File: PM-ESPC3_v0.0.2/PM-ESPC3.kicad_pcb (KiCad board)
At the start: 2 copper layers, 30.5 x 55.9 mm, 15 parts, among them J1 U254-051T-4BH83-S1S, J2 PinHeader_01x13_P2.54_THT_str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, J3 PinHeader_01x01_P2.54_THT_str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, SW1 Button, SW2 Button, SW3 DIP_SW-3P-P2.54-THT-Top, U1 ESP32-C3-WROOM-02U-N4

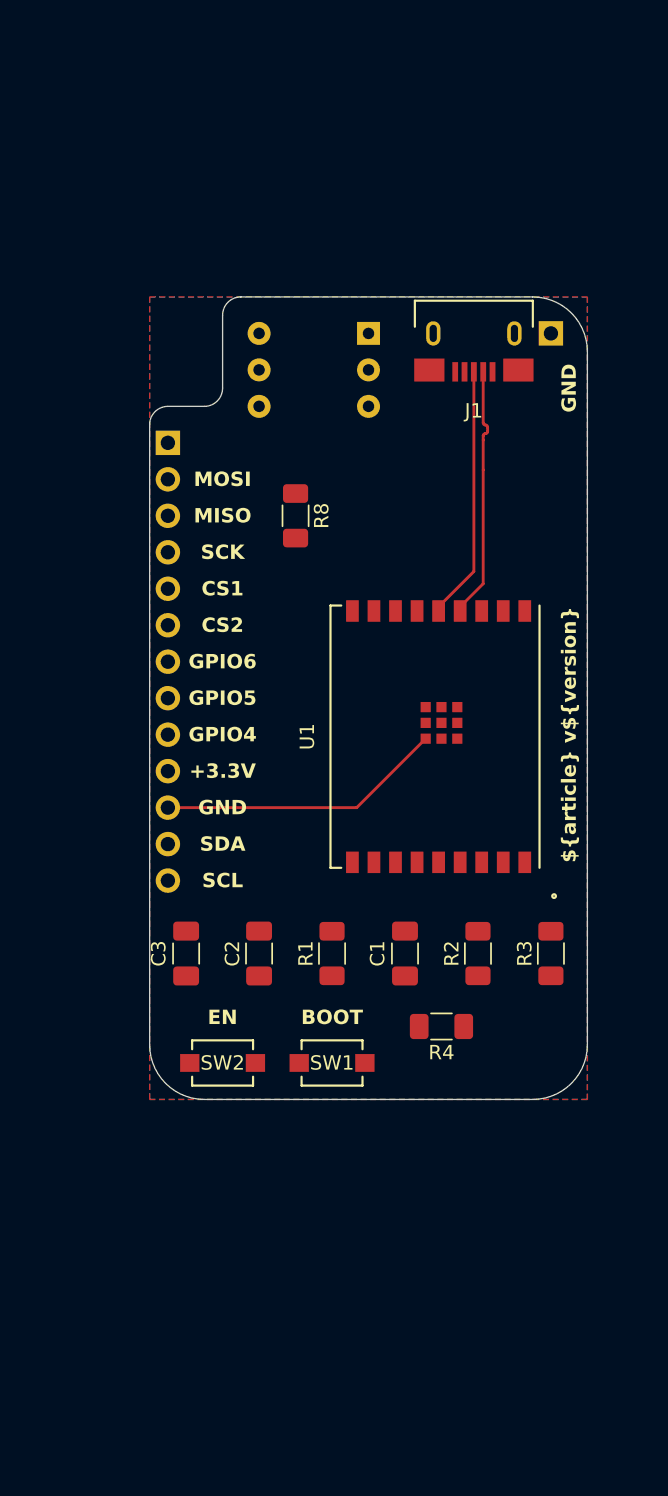
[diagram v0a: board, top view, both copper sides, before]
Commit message: new PM-RQ8
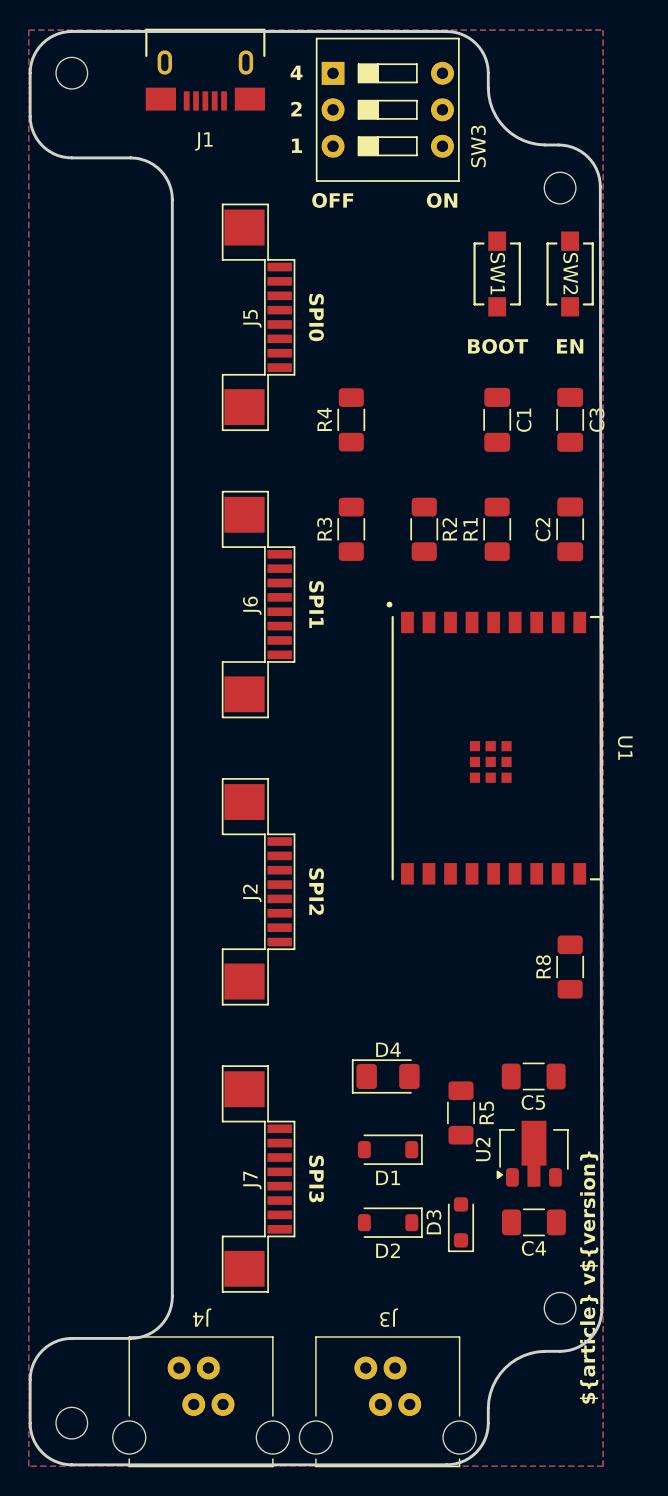
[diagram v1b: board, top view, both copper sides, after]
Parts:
- added C4: 10uF, Capacitor_SMD:C_1206_3216Metric_Pad1.33x1.80mm_HandSolder, F.Cu at (85.2, 133.0)
- added C5: 22uF, Capacitor_SMD:C_1206_3216Metric_Pad1.33x1.80mm_HandSolder, F.Cu at (85.2, 122.9)
- added D1: B5819W, Diode_SMD:D_SOD-123, F.Cu at (75.0, 128.0)
- added D2: B5819W, Diode_SMD:D_SOD-123, F.Cu at (75.0, 133.0)
- added D3: 5A 9.8V 6V, Diode_SMD:D_SOD-323_HandSoldering, F.Cu at (80.1, 133.0)
- added D4: Green, LED_SMD:LED_1206_3216Metric_Pad1.42x1.75mm_HandSolder, F.Cu at (75.0, 122.9)
- added H1: MountingHole, MountingHole:MountingHole_2.2mm_M2, F.Cu at (87.0, 139.0)
- added H2: MountingHole, MountingHole:MountingHole_2.2mm_M2, F.Cu at (53.0, 147.0)
- added H3: MountingHole, MountingHole:MountingHole_2.2mm_M2, F.Cu at (87.0, 61.0)
- added H4: MountingHole, MountingHole:MountingHole_2.2mm_M2, F.Cu at (53.0, 53.0)
- added J4: R-RJ11R04P-A802, kicad_inventree_lib:R-RJ11R04P-A802, F.Cu at (62.0, 148.0)
- added J5: X10B25L08T, kicad_inventree_lib:X10B25L08T, F.Cu at (67.5, 70.0)
- added J6: X10B25L08T, kicad_inventree_lib:X10B25L08T, F.Cu at (67.5, 90.0)
- added J7: X10B25L08T, kicad_inventree_lib:X10B25L08T, F.Cu at (67.5, 130.0)
- added R5: 680R, Resistor_SMD:R_1206_3216Metric_Pad1.30x1.75mm_HandSolder, F.Cu at (80.1, 125.4)
- added U2: CJA1117B-3.3, Package_TO_SOT_SMD:SOT-89-3, F.Cu at (85.2, 127.9)
- J2: value PinHeader_01x13_P2.54_THT_straight -> X10B25L08T; footprint Connector_PinHeader_2.54mm:PinHeader_1x13_P2.54mm_Vertical -> kicad_inventree_lib:X10B25L08T; moved to F.Cu
- J3: value PinHeader_01x01_P2.54_THT_straight -> R-RJ11R04P-A802; footprint Connector_PinHeader_2.54mm:PinHeader_1x01_P2.54mm_Vertical -> kicad_inventree_lib:R-RJ11R04P-A802; moved to F.Cu
- SW3: moved to F.Cu
- moved J3 77.7 mm to (75.0, 148.0)
- moved SW2 60.0 mm to (87.7, 67.0), turned to -90 degrees
- moved SW1 56.1 mm to (82.6, 67.0), turned to -90 degrees
- moved C3 45.8 mm to (87.7, 77.1), turned to 90 degrees
- moved R4 42.7 mm to (72.5, 77.1), turned to 90 degrees
- moved C1 37.7 mm to (82.6, 77.1), turned to 90 degrees
- moved R8 36.8 mm to (87.7, 115.2), turned to 90 degrees
- moved C2 36.6 mm to (87.7, 84.8)
- moved R3 32.6 mm to (72.5, 84.8)
- moved J2 32.2 mm to (67.5, 110.0), turned to -90 degrees
- moved R1 31.7 mm to (82.6, 84.8)
- moved R2 29.8 mm to (77.5, 84.8), turned to -90 degrees
- moved J1 26.6 mm to (63.6, 55.1)
- moved SW3 18.3 mm to (71.2, 53.0), turned to 0 degrees
- moved U1 4.40 mm to (82.6, 100.0), turned to -90 degrees
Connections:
- C2 pad 2: /+3.3V -> +3.3V
- C3 pad 1: /+3.3V -> +3.3V
- J1 pad 1: unconnected-(J1-VBUS-Pad1) -> Net-(D1-A)
- J2 pad 1: unconnected-(J2-Pin_1-Pad1) -> +5V
- J2 pad 2: /GPIO2 -> +3.3V
- J2 pad 3: /GPIO3 -> unconnected-(J2-Pin_3-Pad3)
- J2 pad 4: /GPIO9 -> /MOSI
- J2 pad 5: /GPIO8 -> /MISO
- J2 pad 6: /GPIO7 -> /SCK
- J2 pad 7: /GPIO6 -> /CS2
- J2 pad 8: /GPIO5 -> GND
- J3 pad 1: GND -> Net-(D2-A)
- R1 pad 1: /+3.3V -> +3.3V
- R2 pad 1: /+3.3V -> +3.3V
- R2 pad 2: /GPIO8 -> /A1
- R3 pad 1: /+3.3V -> +3.3V
- R3 pad 2: /GPIO9 -> /A2
- R4 pad 1: /GPIO9 -> /A2
- R8 pad 1: /+3.3V -> +3.3V
- R8 pad 2: /GPIO2 -> /MISO
- SW3 pad 1: /A2 -> +3.3V
- SW3 pad 2: /A1 -> +3.3V
- SW3 pad 3: /A0 -> +3.3V
- SW3 pad 4: /+3.3V -> /A0
- SW3 pad 5: /+3.3V -> /A1
- SW3 pad 6: /+3.3V -> /A2
- U1 pad 1: /+3.3V -> +3.3V
- U1 pad 10: /A2 -> /CS0
- U1 pad 11: /A1 -> /CS1
- U1 pad 12: /A0 -> /CS2
- U1 pad 15: /GPIO3 -> /CS3
- U1 pad 16: /GPIO2 -> /MISO
- U1 pad 3: /GPIO4 -> unconnected-(U1-IO4-Pad3)
- U1 pad 4: /GPIO5 -> /MOSI
- U1 pad 5: /GPIO6 -> /SCK
- U1 pad 6: /GPIO7 -> /A0
- U1 pad 7: /GPIO8 -> /A1
- U1 pad 8: /GPIO9 -> /A2
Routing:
- net GND: track 19.9 -> 0.00 mm
- net /USB_D+: track 17.7 -> 0.00 mm
- net /USB_D-: track 17.6 -> 0.00 mm
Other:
- board size 30.5 x 55.9 mm -> 39.8 x 99.8 mm
- board text added: "1"
- board text added: "2"
- board text added: "4"
- board text added: "OFF"
- board text added: "ON"
- board text added: "SPI0"
- board text added: "SPI1"
- board text added: "SPI2"
- board text added: "SPI3"
- board text removed: "+3.3V"
- board text removed: "CS1"
- board text removed: "CS2"
- board text removed: "GND"
- board text removed: "GPIO4"
- board text removed: "GPIO5"
- board text removed: "GPIO6"
- board text removed: "MISO"
- board text removed: "MOSI"
- board text removed: "SCK"
- board text removed: "SCL"
- board text removed: "SDA"
